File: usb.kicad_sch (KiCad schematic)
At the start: 21 parts, among them J11 USB_C_Receptacle_USB2.0_16P, SW1 SW_Rotary_1x4_MP, SW2 SW_Rotary_1x4_MP

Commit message: footprints
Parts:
- C16, C27: footprint Capacitor_SMD:C_0603_1608Metric -> Capacitor_SMD:C_0201_0603Metric
- R13, R14, R15, R16, R17, R18: footprint (none) -> Resistor_SMD:R_0603_1608Metric
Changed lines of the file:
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@@
 			)
 		)
-		(property "Footprint" ""
+		(property "Footprint" "Resistor_SMD:R_0603_1608Metric"
 			(at 186.69 60.198 90)
 			(effects
@@
 			)
 		)
-		(property "Footprint" ""
+		(property "Footprint" "Resistor_SMD:R_0603_1608Metric"
 			(at 186.69 57.658 90)
 			(effects
@@
 			)
 		)
-		(property "Footprint" ""
+		(property "Footprint" "Resistor_SMD:R_0603_1608Metric"
 			(at 181.61 51.308 90)
 			(effects
@@
 			)
 		)
-		(property "Footprint" "Capacitor_SMD:C_0603_1608Metric"
+		(property "Footprint" "Capacitor_SMD:C_0201_0603Metric"
 			(at 86.0552 52.07 0)
 			(effects
@@
 			)
 		)
-		(property "Footprint" ""
+		(property "Footprint" "Resistor_SMD:R_0603_1608Metric"
 			(at 181.61 46.228 90)
 			(effects
@@
 			)
 		)
-		(property "Footprint" ""
+		(property "Footprint" "Resistor_SMD:R_0603_1608Metric"
 			(at 181.61 48.768 90)
 			(effects
@@
 			)
 		)
-		(property "Footprint" ""
+		(property "Footprint" "Resistor_SMD:R_0603_1608Metric"
 			(at 186.69 62.738 90)
 			(effects
@@
 			)
 		)
-		(property "Footprint" "Capacitor_SMD:C_0603_1608Metric"
+		(property "Footprint" "Capacitor_SMD:C_0201_0603Metric"
 			(at 96.2152 52.07 0)
 			(effects

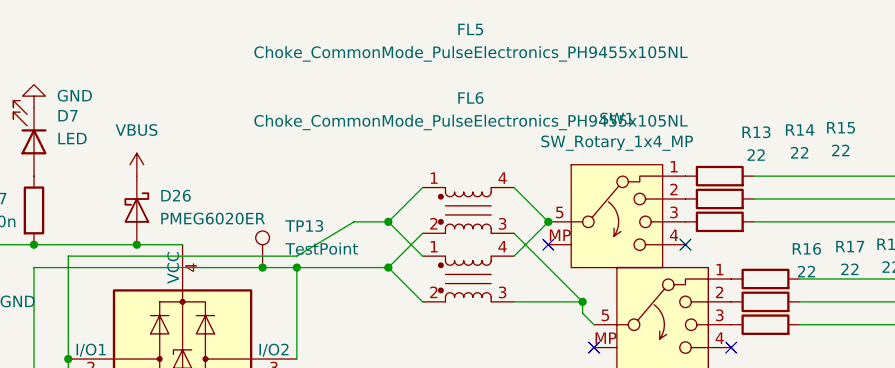
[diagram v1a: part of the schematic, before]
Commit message: i fogro
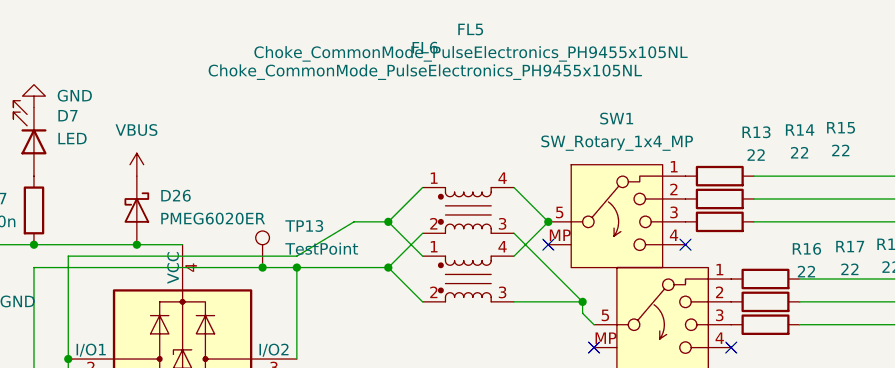
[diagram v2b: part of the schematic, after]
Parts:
- SW1, SW2: footprint (none) -> Rotary_Encoder:RotaryEncoder_Alps_EC12E_Vertical_H20mm
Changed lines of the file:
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@@
 			)
 		)
-		(property "Footprint" ""
+		(property "Footprint" "Rotary_Encoder:RotaryEncoder_Alps_EC12E_Vertical_H20mm"
 			(at 175.26 71.12 0)
 			(effects
@@
 		(dnp no)
 		(property "Reference" "FL6"
-			(at 153.924 35.814 0)
+			(at 148.844 30.226 0)
 			(effects
 				(font
@@
 		)
 		(property "Value" "Choke_CommonMode_PulseElectronics_PH9455x105NL"
-			(at 153.924 38.354 0)
+			(at 148.844 32.766 0)
 			(effects
 				(font
@@
 			)
 		)
-		(property "Footprint" ""
+		(property "Footprint" "Rotary_Encoder:RotaryEncoder_Alps_EC12E_Vertical_H20mm"
 			(at 170.18 59.69 0)
 			(effects

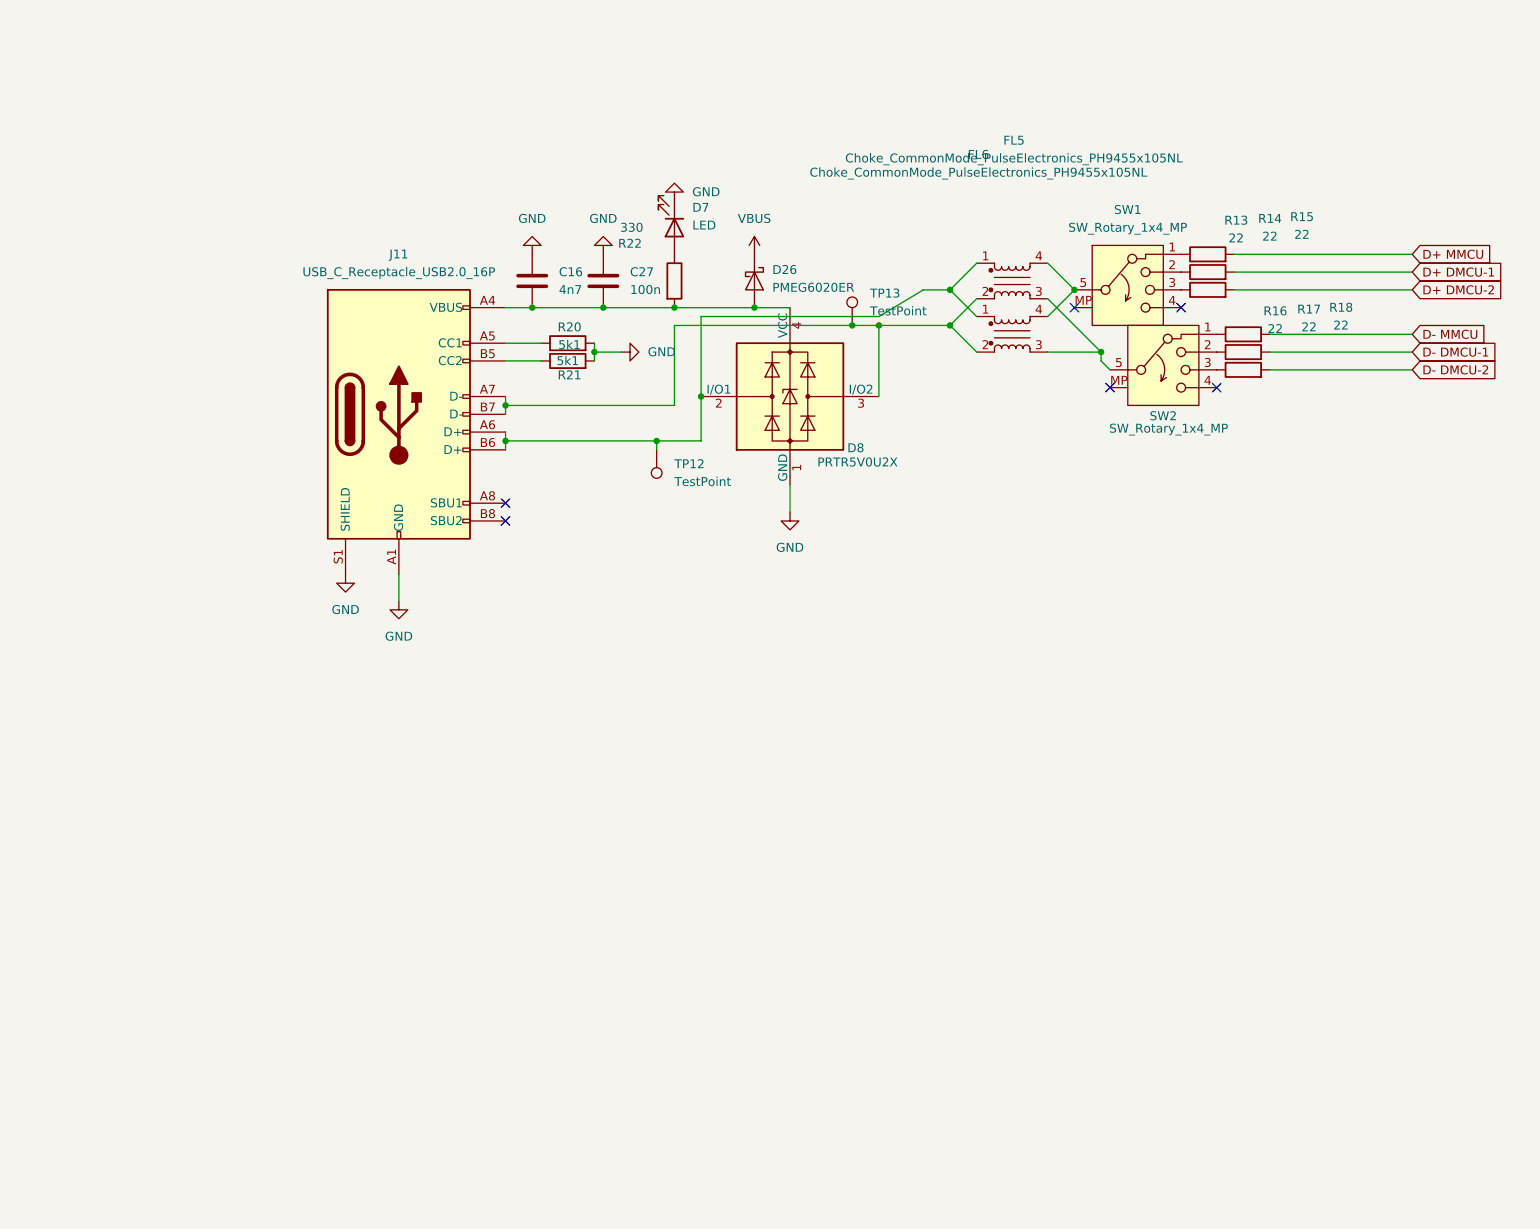
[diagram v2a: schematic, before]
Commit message: started pcb
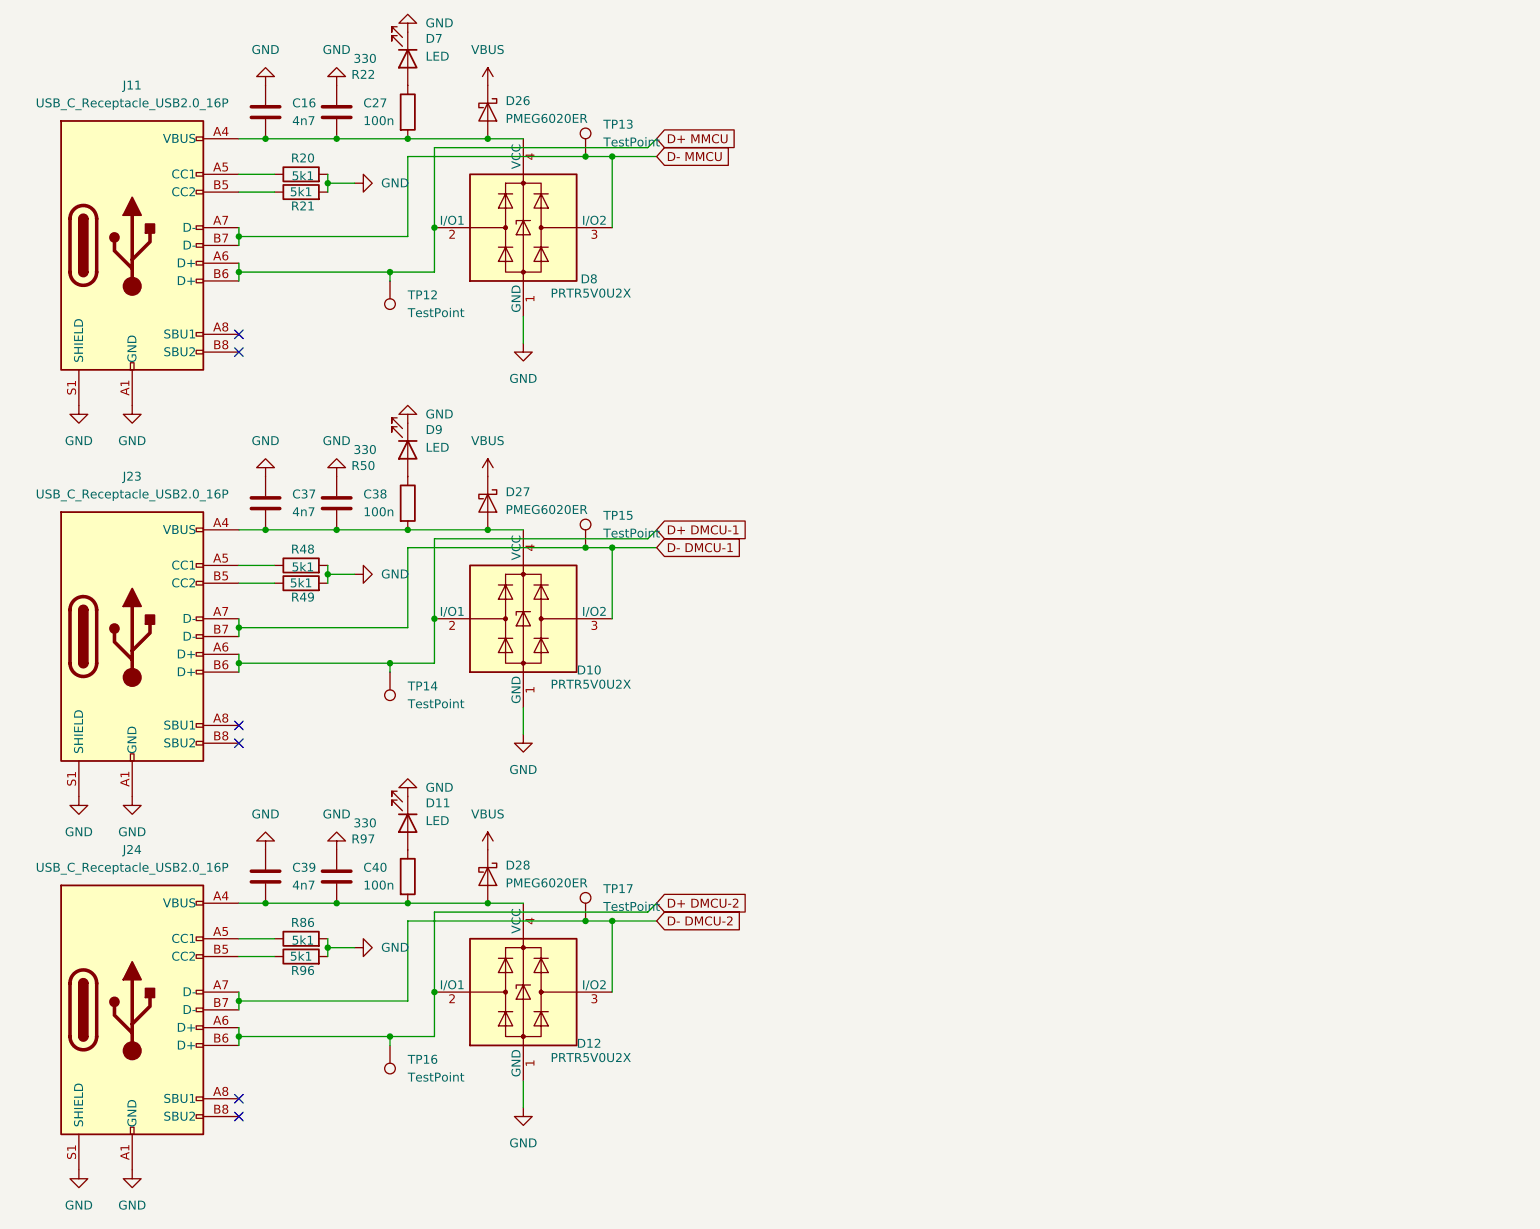
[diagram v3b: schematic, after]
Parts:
- removed FL5, FL6: Choke_CommonMode_PulseElectronics_PH9455x105NL, Inductor_THT:L_CommonMode_PulseElectronics_PH9455x105NL_1, symbol Filter:Choke_CommonMode_PulseElectronics_PH9455x105NL
- removed R13, R14, R15, R16, R17, R18: 22, Resistor_SMD:R_0603_1608Metric, symbol Device:R
- removed SW1, SW2: SW_Rotary_1x4_MP, Rotary_Encoder:RotaryEncoder_Alps_EC12E_Vertical_H20mm, symbol Switch:SW_Rotary_1x4_MP
- added C37, C39: 4n7, Capacitor_SMD:C_0603_1608Metric, symbol Device:C
- added C38, C40: 100n, Capacitor_SMD:C_0603_1608Metric, symbol Device:C
- added D10, D12: PRTR5V0U2X, Package_TO_SOT_SMD:SOT-143, symbol Power_Protection:PRTR5V0U2X
- added D11, D9: LED, LED_SMD:LED_0603_1608Metric, symbol Device:LED
- added D27, D28: PMEG6020ER, Diode_SMD:Nexperia_CFP3_SOD-123W, symbol Diode:PMEG6020ER
- added J23, J24: USB_C_Receptacle_USB2.0_16P, Connector_USB:USB_C_Receptacle_Amphenol_124019772112A, symbol Connector:USB_C_Receptacle_USB2.0_16P
- added R48, R49, R86, R96: 5k1, Resistor_SMD:R_0603_1608Metric, symbol Device:R
- added R50, R97: 330, Resistor_SMD:R_0603_1608Metric, symbol Device:R
- added TP14, TP15, TP16, TP17: TestPoint, TestPoint:TestPoint_Pad_1.0x1.0mm, symbol Connector:TestPoint
- C16, C27: footprint Capacitor_SMD:C_0201_0603Metric -> Capacitor_SMD:C_0603_1608Metric
- D7: footprint LED_SMD:LED_0201_0603Metric -> LED_SMD:LED_0603_1608Metric
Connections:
- net D+ DMCU-1: now also D10.2 (I/O1), J23.A6 (D+), J23.B6 (D+), TP14.1
- net D+ DMCU-2: now also D12.2 (I/O1), J24.A6 (D+), J24.B6 (D+), TP16.1
- net D+ MMCU: now also D8.2 (I/O1), J11.A6 (D+), J11.B6 (D+), TP12.1
- net D- DMCU-1: now also D10.3 (I/O2), J23.A7 (D-), J23.B7 (D-), TP15.1
- net D- DMCU-2: now also D12.3 (I/O2), J24.A7 (D-), J24.B7 (D-), TP17.1
- net D- MMCU: now also D8.3 (I/O2), J11.A7 (D-), J11.B7 (D-), TP13.1
- net GND: now also C37.1, C38.1, C39.1, C40.1, D10.1 (GND), D11.1 (K), D12.1 (GND), D9.1 (K), J23.A1 (GND), J23.A12 (GND), J23.B1 (GND), J23.B12 (GND), J23.S1 (SHIELD), J24.A1 (GND), J24.A12 (GND), J24.B1 (GND), J24.B12 (GND), J24.S1 (SHIELD), R48.2, R49.2, R86.2, R96.2
- net VBUS: now also D27.1 (K), D28.1 (K)
- new net: C39.2, C40.2, D12.4 (VCC), D28.2 (A), J24.A4 (VBUS), J24.A9 (VBUS), J24.B4 (VBUS), J24.B9 (VBUS), R97.2
- new net: C37.2, C38.2, D10.4 (VCC), D27.2 (A), J23.A4 (VBUS), J23.A9 (VBUS), J23.B4 (VBUS), J23.B9 (VBUS), R50.2
- new net: D11.2 (A), R97.1
- new net: J24.B5 (CC2), R96.1
- new net: J23.A5 (CC1), R48.1
- new net: J23.B5 (CC2), R49.1
- new net: J24.A5 (CC1), R86.1
- new net: D9.2 (A), R50.1
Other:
- moved on the sheet: C16, C27, D26, D7, D8, J11, R20, R21, R22, TP12, TP13

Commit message: new usb, move micro sd, redo boost converter (pls find a place on the pcb tomorrow)
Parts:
- J11, J23, J24: footprint Connector_USB:USB_C_Receptacle_Amphenol_124019772112A -> Connector_USB:USB_C_Receptacle_GCT_USB4105-xx-A_16P_TopMnt_Horizontal
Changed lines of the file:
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@@
 			)
 		)
-		(property "Footprint" "Connector_USB:USB_C_Receptacle_Amphenol_124019772112A"
+		(property "Footprint" "Connector_USB:USB_C_Receptacle_GCT_USB4105-xx-A_16P_TopMnt_Horizontal"
 			(at 31.75 99.06 0)
 			(effects
@@
 			)
 		)
-		(property "Footprint" "Connector_USB:USB_C_Receptacle_Amphenol_124019772112A"
+		(property "Footprint" "Connector_USB:USB_C_Receptacle_GCT_USB4105-xx-A_16P_TopMnt_Horizontal"
 			(at 31.75 152.4 0)
 			(effects
@@
 			)
 		)
-		(property "Footprint" "Connector_USB:USB_C_Receptacle_Amphenol_124019772112A"
+		(property "Footprint" "Connector_USB:USB_C_Receptacle_GCT_USB4105-xx-A_16P_TopMnt_Horizontal"
 			(at 31.75 43.18 0)
 			(effects
